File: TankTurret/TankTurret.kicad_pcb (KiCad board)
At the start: 2 copper layers, 35 x 60 mm, 59 parts, among them J1 Conn_01x04_Socket, J2 USB_C_Receptacle_USB2.0_16P, J3 Camera, Q1 MMBT3904, SW1 SW_Push, SW2 SW_Push, U1 ESP32-S3-WROOM-1, U3 ME6211C28M5G, U4 LN1234B132MR-G

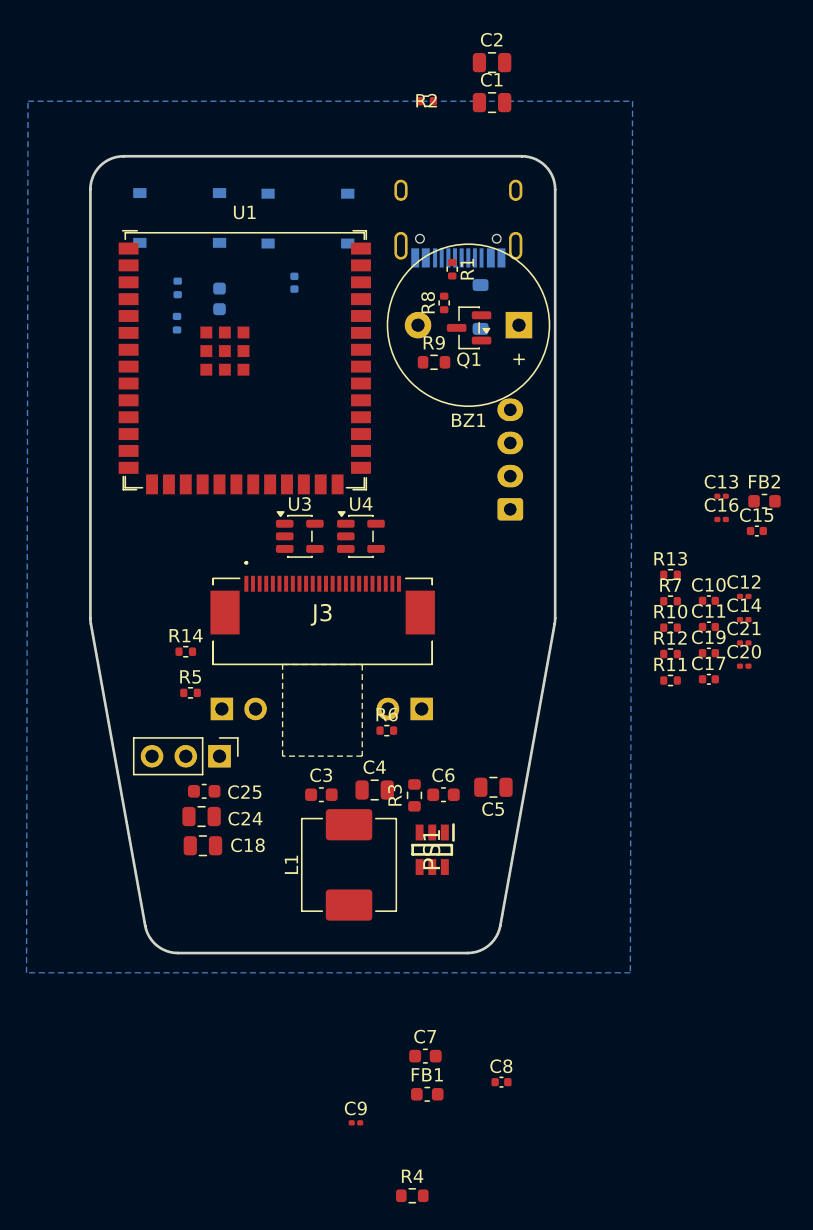
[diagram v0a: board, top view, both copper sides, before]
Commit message: Signed-off-by: SMAUG\Pete <pwbrophy@gmail.com>
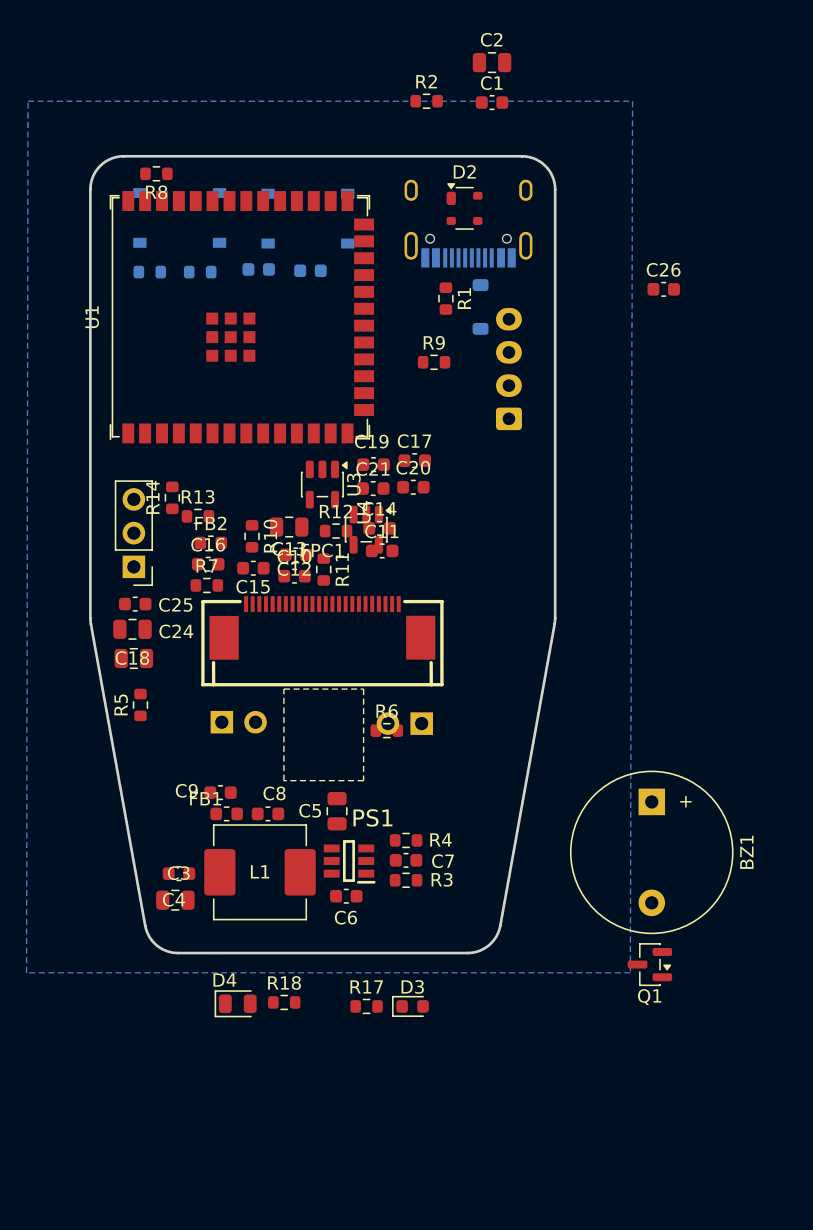
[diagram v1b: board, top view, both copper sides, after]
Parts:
- removed J3: Camera, Jushuo:AFC07-S24ECA-00_flux
- added C26: 100nF, Capacitor_SMD:C_0603_1608Metric, F.Cu at (97.0, 51.3)
- added D2: PRTR5V0U2X, Package_TO_SOT_SMD:SOT-143, F.Cu at (82.0, 45.2)
- added D3: LED, LED_SMD:LED_0603_1608Metric, F.Cu at (78.1, 105.3)
- added D4: LED, LED_SMD:LED_0805_2012Metric, F.Cu at (64.9, 105.1)
- added FPC1: AFC07-S24ECA-00, EasyEDA2Kicad:FPC-SMD_AFC07-S24ECA-00, F.Cu at (71.3, 76.3)
- added R17: 10k, Resistor_SMD:R_0603_1608Metric, F.Cu at (74.6, 105.3)
- added R18: 1k, Resistor_SMD:R_0603_1608Metric, F.Cu at (68.4, 105.0)
- C1: footprint Capacitor_SMD:C_0805_2012Metric -> Capacitor_SMD:C_0603_1608Metric
- C10, C11, C15, C17, C19, C22, C8: footprint Capacitor_SMD:C_0402_1005Metric -> Capacitor_SMD:C_0603_1608Metric
- C12, C14, C16, C20, C21, C9: footprint Capacitor_SMD:C_0201_0603Metric -> Capacitor_SMD:C_0603_1608Metric
- C13: footprint Capacitor_SMD:C_0201_0603Metric -> Capacitor_SMD:C_0805_2012Metric
- C23: value 1.0uF -> 1uF
- R1, R10, R11, R12, R13, R14, R15, R16, R2, R5, R6, R7, R8: footprint Resistor_SMD:R_0402_1005Metric -> Resistor_SMD:R_0603_1608Metric
- moved Q1 49.8 mm to (96.0, 102.2)
- moved FB2 41.8 mm to (62.9, 70.4)
- moved C16 38.8 mm to (62.7, 72.0)
- moved C15 38.0 mm to (66.1, 72.3), turned to 180 degrees
- moved BZ1 37.3 mm to (96.1, 89.9), turned to -90 degrees
- moved R13 35.9 mm to (61.9, 68.4)
- moved R7 34.9 mm to (62.6, 73.6)
- moved C12 33.9 mm to (69.3, 71.3), turned to 180 degrees
- moved C13 32.6 mm to (68.8, 69.2), turned to 180 degrees
- moved R10 32.3 mm to (66.0, 69.9), turned to -90 degrees
- moved C10 31.3 mm to (69.2, 72.9)
- moved C21 30.3 mm to (75.1, 66.3)
- moved C19 29.0 mm to (75.2, 64.5)
- moved C20 28.3 mm to (78.2, 66.2)
- moved C14 28.3 mm to (75.6, 69.3)
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- renumbered CON_IR_LED_1 to J4, CON_IR_LED_2 to J5, CON_STATUS_LED1 to J6
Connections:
- net +5V_USB renamed /+5V_USB
- net USB_D+ renamed /USB_D+
- net USB_D- renamed /USB_D-
- R15 pad 1: +3V3_CLEAN -> +3V3
- R16 pad 1: +3V3_CLEAN -> +3V3
- U1 pad 2: +3V3_CLEAN -> +3V3
- U1 pad 25: unconnected-(U1-GPIO48/SPICLK_N/SUBSPICLK_N_DIFF-Pad25) -> /GPIO48
